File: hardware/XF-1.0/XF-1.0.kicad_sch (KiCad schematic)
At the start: 9 parts

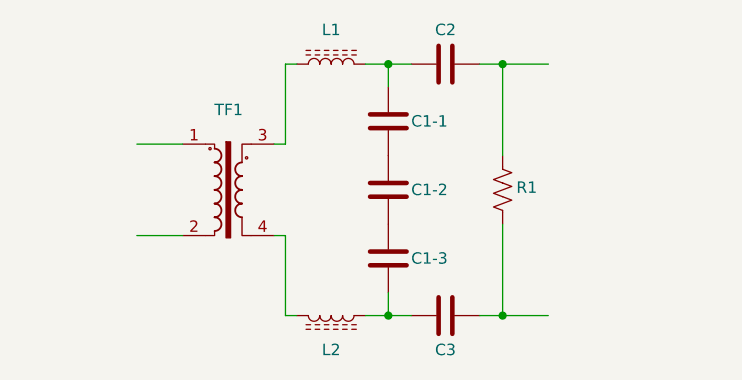
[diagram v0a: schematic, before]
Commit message: modified:   Ferrite Transformer Calculation.xlsx 	modified:   README.md 	deleted:    hardware/XF-1.0/XF-1.0-backups/XF-1.0-2025-07-15_095716.zip 	new file:   hardware/XF-1.0/XF-1.0-backups/XF-1.0-2025-07-15_145509.zip 	new file:   hardware/XF-1.0/XF-1.0-backups/XF-1.0-2025-07-15_150114.zip 	new file:   hardware/XF-1.0/XF-1.0-backups/XF-1.0-2025-07-15_150614.zip 	new file:   hardware/XF-1.0/XF-1.0-backups/XF-1.0-2025-07-15_151503.zip 	new file:   hardware/XF-1.0/XF-1.0-backups/XF-1.0-2025-07-15_152320.zip 	new file:   hardware/XF-1.0/XF-1.0-backups/XF-1.0-2025-07-15_154638.zip 	modified:   hardware/XF-1.0/XF-1.0.kicad_pcb 	modified:   hardware/XF-1.0/XF-1.0.kicad_prl 	modified:   hardware/XF-1.0/XF-1.0.kicad_pro 	modified:   hardware/XF-1.0/XF-1.0.kicad_sch 	modified:   hardware/XF-1.0/_autosave-XF-1.0.kicad_sch 	modified:   hardware/XF-1.0/fp-info-cache
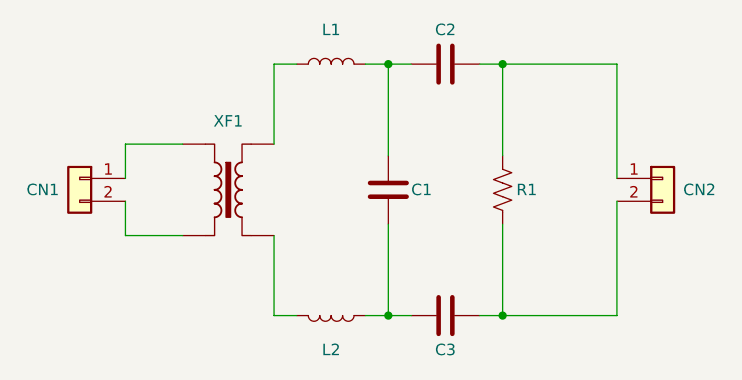
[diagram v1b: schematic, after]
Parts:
- removed C1-2, C1-3: 1nF, Capacitor_THT:C_Rect_L13.0mm_W8.0mm_P10.00mm_FKS3_FKP3_MKS4, symbol Device:C
- removed L1, L2: ~, Transformer_THT:Inductor-EE25, symbol Device:L_Ferrite
- removed TF1: ~, Transformer_THT:EE35-1P-1S-Vertical-2143, symbol Transformer:ER35-1P-1S
- added CN1, CN2: Conn_01x02, Connector_Molex:Molex_KK-396_5273-03A_1x03_P3.96mm_Vertical_2, symbol Connector_Generic:Conn_01x02
- added L1, L2: 29µH, Inductor_THT:L_Radial_Multilayer_D8.0mm_P12.70mm, symbol Device:L
- added XF1: ~, Transformer_THT:Transformer_Toroid_Horizontal_OD40_ID23_H15, symbol Transformer:TRANSF1
- C1: renamed from C1-1; value 1nF -> 2.7nF
- R1: value R_US -> RBTL
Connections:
- net at C3.1: now also C1.2, L2.2
- net at C3.2, R1.2: now also CN2.2 (Pin_2)
- net at C1.1, C2.1: now also L1.2
- net at C2.2, R1.1: now also CN2.1 (Pin_1)
- new net: L1.1, XF1.4
- new net: L2.1, XF1.3
- new net: CN1.1 (Pin_1), XF1.1
- new net: CN1.2 (Pin_2), XF1.2
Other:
- moved on the sheet: C1
